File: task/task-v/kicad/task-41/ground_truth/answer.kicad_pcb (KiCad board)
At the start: 2 copper layers, 40 x 35 mm, 3 parts

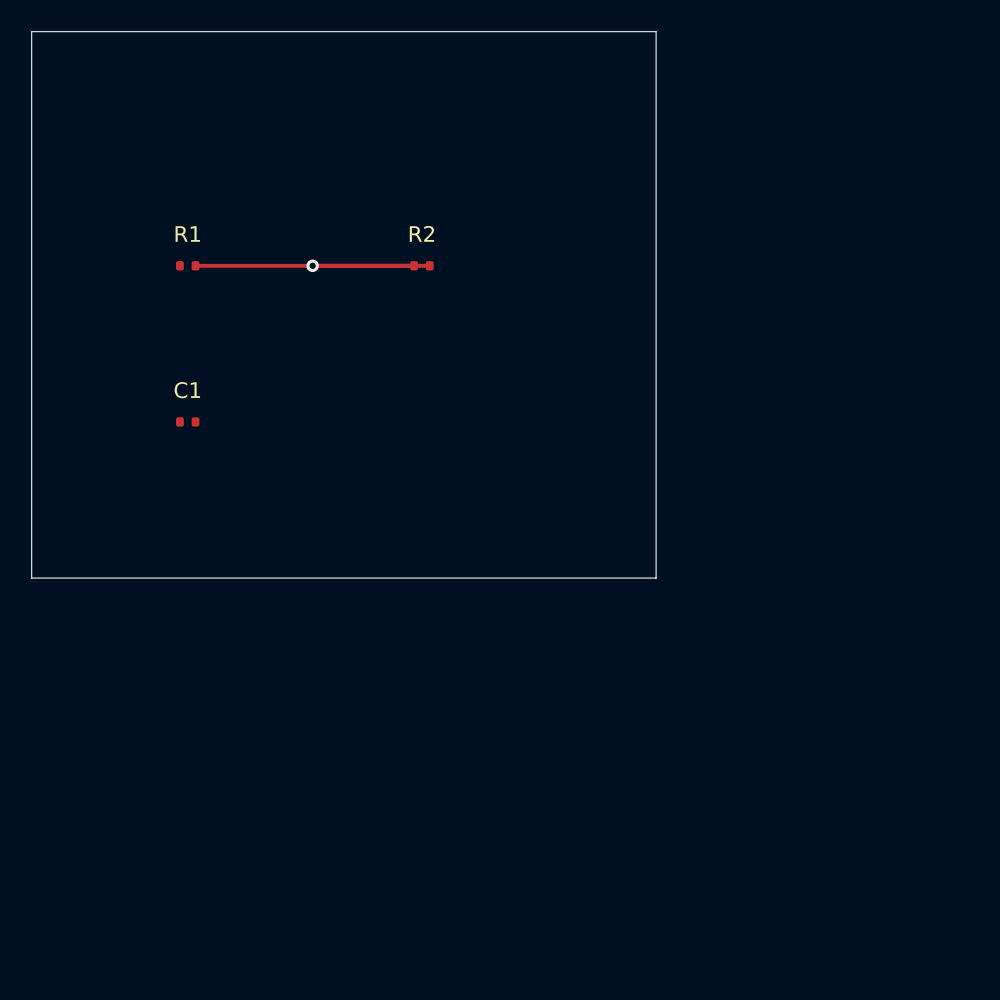
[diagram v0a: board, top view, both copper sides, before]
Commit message: Refine engineering task metadata and instructions
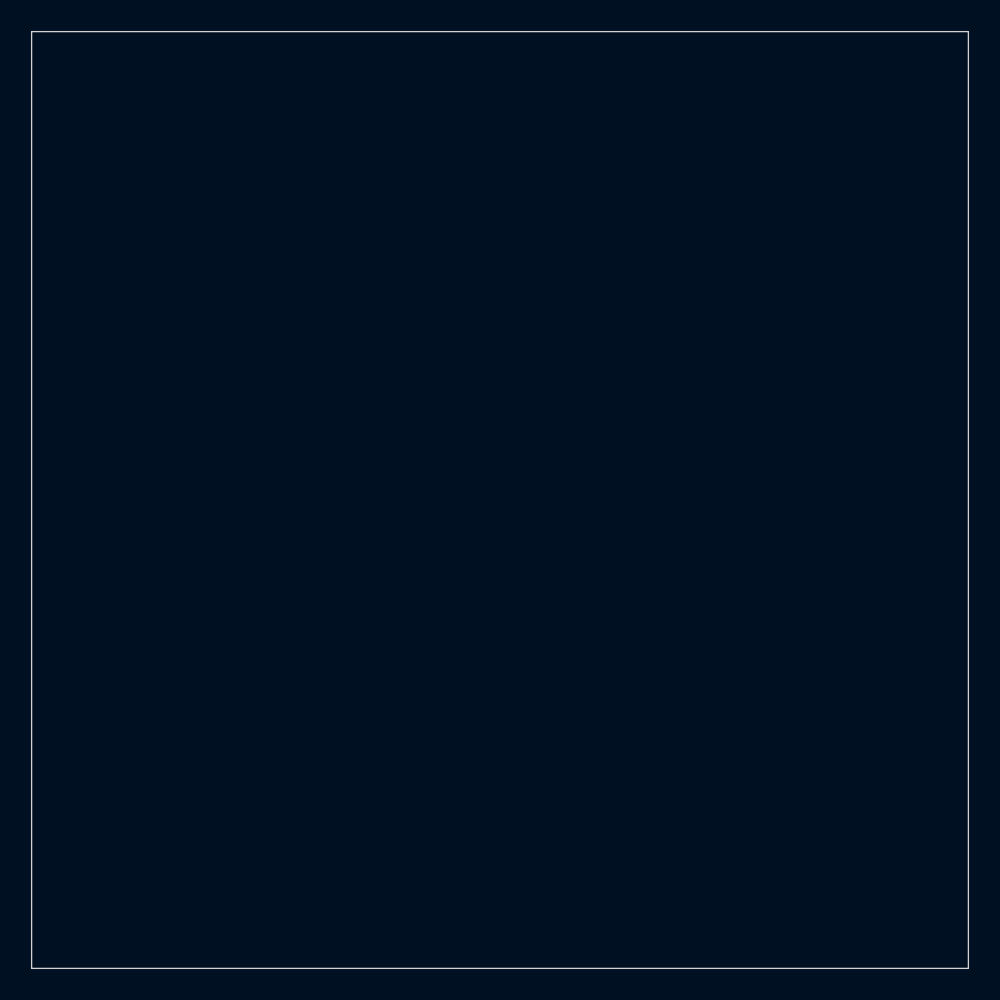
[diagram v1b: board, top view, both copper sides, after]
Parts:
- removed C1: 100n, Capacitor_SMD:C_0402
- removed R1, R2: 10k, Resistor_SMD:R_0402
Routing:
- net SIG_A: track 21.5 -> 0.00 mm, vias 1 -> 0
- added copper zone on In1.Cu, net +3V3
- added copper zone on In1.Cu, net GND
- removed copper zone on F.Cu, net GND
- removed copper zone on F.Cu, net SIG_A
- removed copper zone on F.Cu, net VCC
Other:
- board size 40 x 35 mm -> 60 x 60 mm
- copper layers 2 -> 3
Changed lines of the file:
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@@
   (layers
     (0 "F.Cu" signal)
+    (1 "In1.Cu" power)
     (31 "B.Cu" signal)
     (36 "B.SilkS" user "B.Silkscreen")
@@
   (net 0 "")
   (net 1 "GND")
-  (net 2 "VCC")
-  (net 3 "SIG_A")
-  (net 4 "NC1")
-  (footprint "Resistor_SMD:R_0402"
-    (layer "F.Cu")
-    (at 10 15)
-    (property "Reference" "R1" (at 0 -2) (layer "F.SilkS") (effects (font (size 1 1) (thickness 0.15))))
-    (property "Value" "10k" (at 0 2) (layer "F.Fab") (effects (font (size 1 1) (thickness 0.15))))
-    (pad "1" smd roundrect (at -0.5 0) (size 0.5 0.6) (layers "F.Cu" "F.Paste" "F.Mask") (roundrect_rratio 0.25) (net 3 "SIG_A"))
-    (pad "2" smd roundrect (at 0.5 0) (size 0.5 0.6) (layers "F.Cu" "F.Paste" "F.Mask") (roundrect_rratio 0.25) (net 3 "SIG_A"))
-  )
-  (footprint "Resistor_SMD:R_0402"
-    (layer "F.Cu")
-    (at 25 15)
-    (property "Reference" "R2" (at 0 -2) (layer "F.SilkS") (effects (font (size 1 1) (thickness 0.15))))
-    (property "Value" "10k" (at 0 2) (layer "F.Fab") (effects (font (size 1 1) (thickness 0.15))))
-    (pad "1" smd roundrect (at -0.5 0) (size 0.5 0.6) (layers "F.Cu" "F.Paste" "F.Mask") (roundrect_rratio 0.25) (net 3 "SIG_A"))
-    (pad "2" smd roundrect (at 0.5 0) (size 0.5 0.6) (layers "F.Cu" "F.Paste" "F.Mask") (roundrect_rratio 0.25) (net 1 "GND"))
-  )
-  (footprint "Capacitor_SMD:C_0402"
-    (layer "F.Cu")
-    (at 10 25)
-    (property "Reference" "C1" (at 0 -2) (layer "F.SilkS") (effects (font (size 1 1) (thickness 0.15))))
-    (property "Value" "100n" (at 0 2) (layer "F.Fab") (effects (font (size 1 1) (thickness 0.15))))
-    (pad "1" smd roundrect (at -0.5 0) (size 0.5 0.6) (layers "F.Cu" "F.Paste" "F.Mask") (roundrect_rratio 0.25) (net 2 "VCC"))
-    (pad "2" smd roundrect (at 0.5 0) (size 0.5 0.6) (layers "F.Cu" "F.Paste" "F.Mask") (roundrect_rratio 0.25) (net 1 "GND"))
-  )
-  (segment (start 10.5 15) (end 24.5 15) (width 0.25) (layer "F.Cu") (net 3))
-  (segment (start 25.5 15) (end 18 15) (width 0.25) (layer "F.Cu") (net 3))
-  (via (at 18 15) (size 0.8) (drill 0.4) (layers "F.Cu" "B.Cu") (net 3))
-  (gr_rect (start 0 0) (end 40 35) (layer "Edge.Cuts") (width 0.05))
-  (zone
-    (net 3)
-    (net_name "SIG_A")
-    (layer "F.Cu")
-    (name "TEARDROP_SIG_A_10_15")
-    (hatch none 0.508)
-    (connect_pads (clearance 0.1))
-    (min_thickness 0.1)
-    (teardrop yes)
-    (fill yes)
-  )
-  (zone
-    (net 3)
-    (net_name "SIG_A")
-    (layer "F.Cu")
-    (name "TEARDROP_SIG_A_10_15")
-    (hatch none 0.508)
-    (connect_pads (clearance 0.1))
-    (min_thickness 0.1)
-    (teardrop yes)
-    (fill yes)
-  )
-  (zone
-    (net 3)
-    (net_name "SIG_A")
-    (layer "F.Cu")
-    (name "TEARDROP_SIG_A_24_15")
-    (hatch none 0.508)
-    (connect_pads (clearance 0.1))
-    (min_thickness 0.1)
-    (teardrop yes)
-    (fill yes)
-  )
+  (net 2 "+3V3")
   (zone
     (net 1)
     (net_name "GND")
-    (layer "F.Cu")
-    (name "TEARDROP_GND_26_15")
-    (hatch none 0.508)
-    (connect_pads (clearance 0.1))
-    (min_thickness 0.1)
-    (teardrop yes)
-    (fill yes)
+    (layer "In1.Cu")
+    (name "GND_PLANE")
+    (priority 0)
+    (hatch edge 0.508)
+    (connect_pads (clearance 0.5))
+    (min_thickness 0.25)
+    (fill yes (thermal_gap 0.5) (thermal_bridge_width 0.5))
+    (polygon (pts (xy 0 0) (xy 60 0) (xy 60 60) (xy 0 60)))
   )
   (zone
     (net 2)
-    (net_name "VCC")
-    (layer "F.Cu")
-    (name "TEARDROP_VCC_10_25")
-    (hatch none 0.508)
-    (connect_pads (clearance 0.1))
-    (min_thickness 0.1)
-    (teardrop yes)
-    (fill yes)
+    (net_name "+3V3")
+    (layer "In1.Cu")
+    (name "V33_ZONE")
+    (priority 10)
+    (hatch edge 0.508)
+    (connect_pads (clearance 0.5))
+    (min_thickness 0.25)
+    (fill yes (thermal_gap 0.5) (thermal_bridge_width 0.5))
+    (polygon (pts (xy 0 0) (xy 30 0) (xy 30 30) (xy 0 30)))
   )
-  (zone
-    (net 1)
-    (net_name "GND")
-    (layer "F.Cu")
-    (name "TEARDROP_GND_10_25")
-    (hatch none 0.508)
-    (connect_pads (clearance 0.1))
-    (min_thickness 0.1)
-    (teardrop yes)
-    (fill yes)
-  )
-  (zone
-    (net 3)
-    (net_name "SIG_A")
-    (layer "F.Cu")
-    (name "TEARDROP_SIG_A_18_15")
-    (hatch none 0.508)
-    (connect_pads (clearance 0.1))
-    (min_thickness 0.1)
-    (teardrop yes)
-    (fill yes)
-  )
+  (gr_rect (start 0 0) (end 60 60) (layer "Edge.Cuts") (width 0.05))
 )
